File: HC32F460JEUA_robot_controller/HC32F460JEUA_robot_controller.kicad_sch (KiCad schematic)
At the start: 13 parts, among them CN1 XT30PW-M, U1 HC32F460JEUA-QFN48TR, U3 LMR51450SDRRR, U4 CH343P, U5 TJA1051TK-3

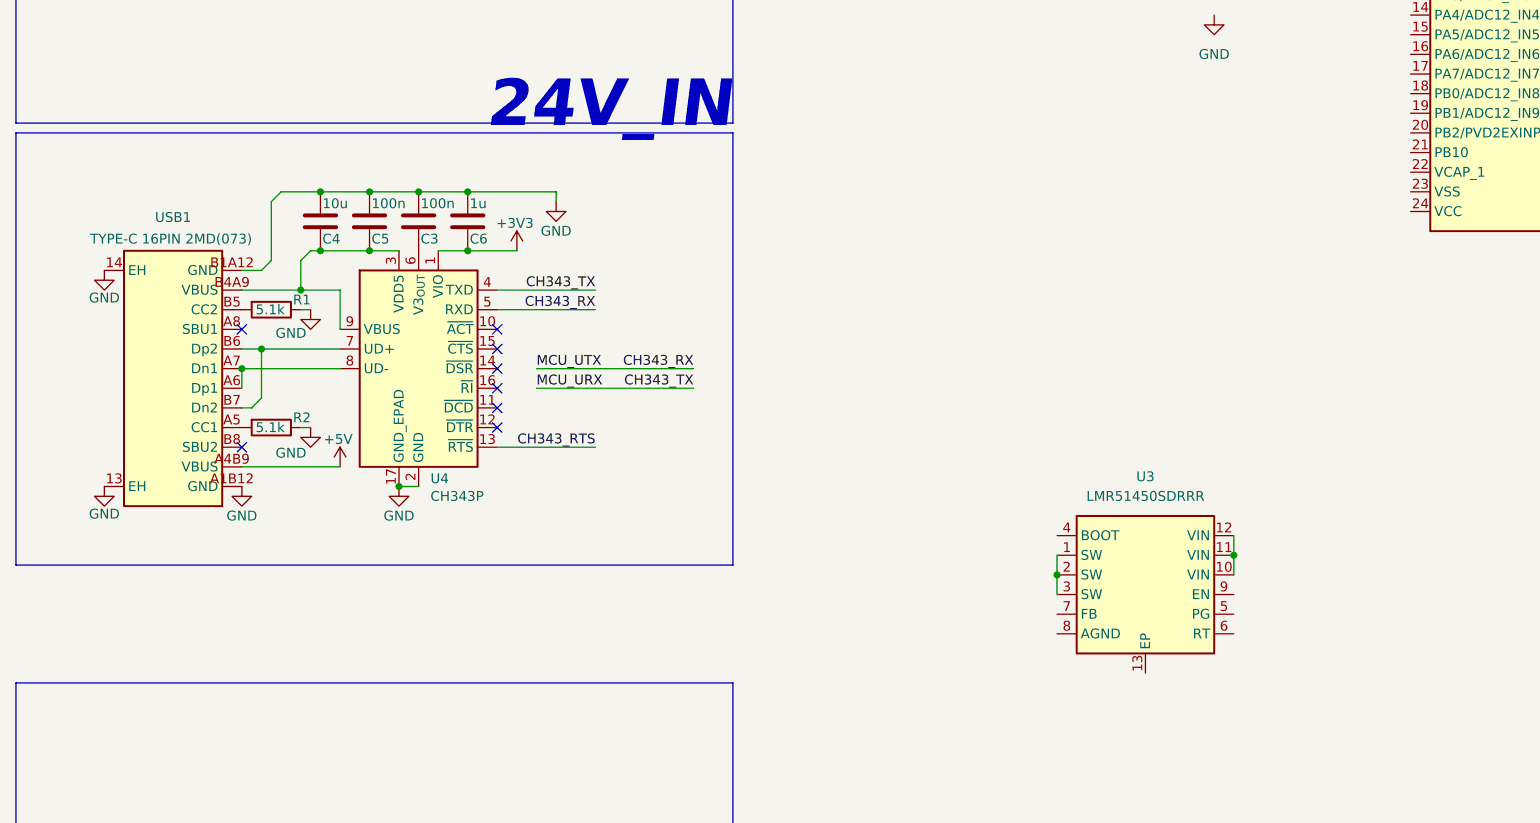
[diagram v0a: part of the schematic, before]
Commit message: Update README to reflect project.
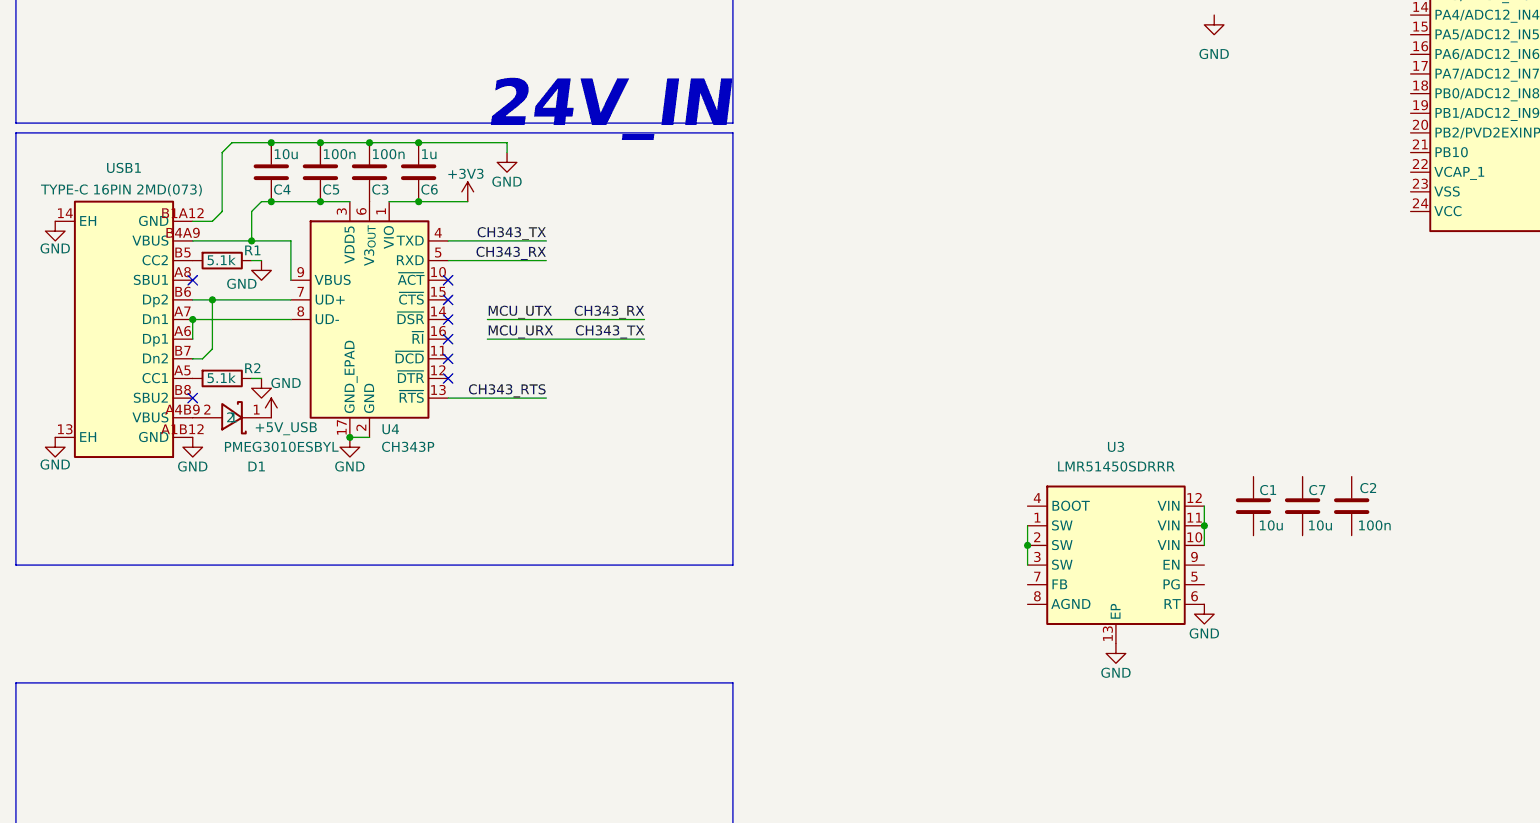
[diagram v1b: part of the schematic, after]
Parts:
- added C1, C7: 10u, Capacitor_SMD:C_0603_1608Metric, symbol Library:C0603
- added C2: 100n, Capacitor_SMD:C_0402_1005Metric, symbol Library:C0402
- added D1: PMEG3010ESBYL, Library:SOD993_L1.0-W0.6-LS1.0-RD, symbol Library:PMEG3010ESBYL
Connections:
- net GND: now also U3.13 (EP), U3.6 (RT)
- net +5V: no longer names the net of USB1.A4B9 (VBUS)
- net +5V: now also D1.2
- new net +5V_USB: D1.1
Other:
- moved on the sheet: C3, C4, C5, C6, R1, R2, U3, U4, USB1
